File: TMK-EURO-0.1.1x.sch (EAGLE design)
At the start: 43 parts, among them IC1 TL082P, U2 IN, U5 IN, U6 IN, U7 THONKICONNOLD, X1 057-010-1

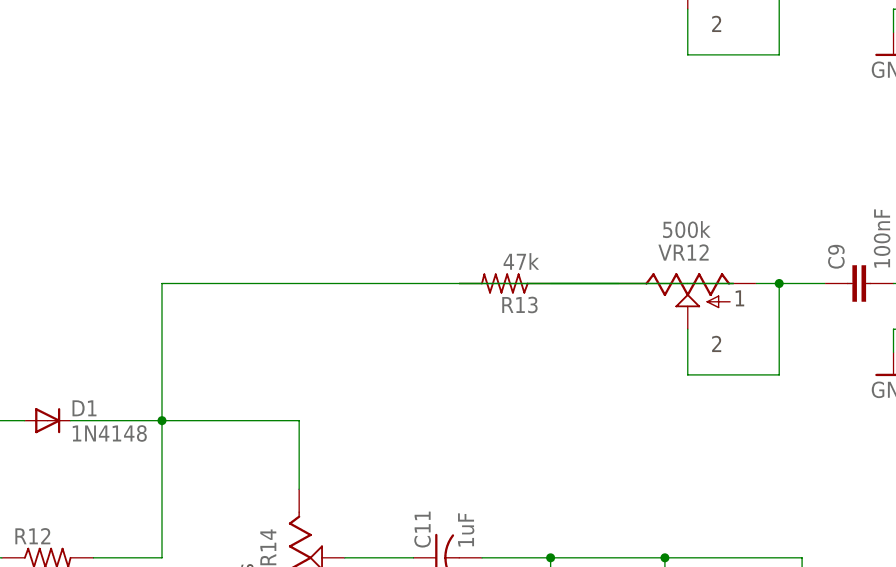
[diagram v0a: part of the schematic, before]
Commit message: Nets netjes
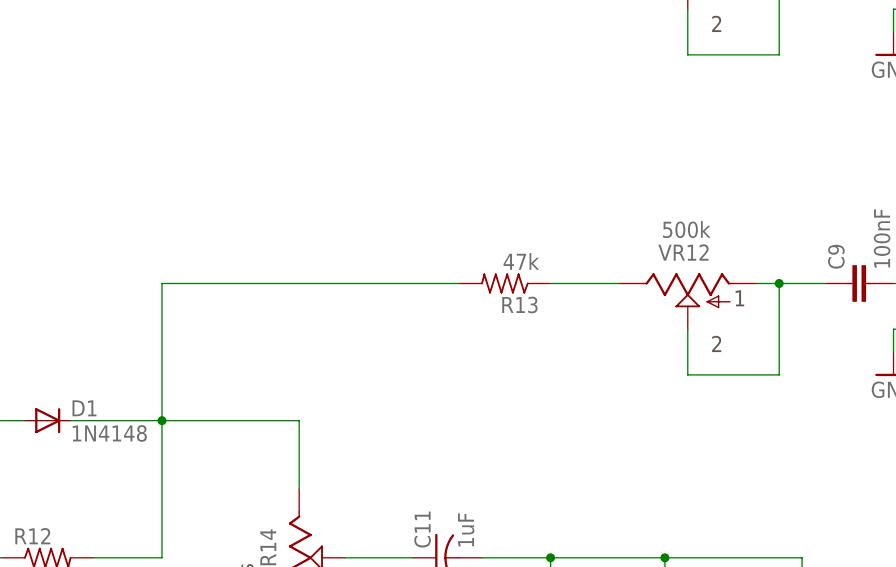
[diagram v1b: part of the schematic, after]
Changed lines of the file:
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@@
 <junction x="208.28" y="116.84"/>
 <wire x1="208.28" y1="116.84" x2="208.28" y2="132.08" width="0.1524" layer="91"/>
-<wire x1="208.28" y1="132.08" x2="246.38" y2="132.08" width="0.1524" layer="91"/>
-<wire x1="246.38" y1="132.08" x2="266.7" y2="132.08" width="0.1524" layer="91"/>
-<wire x1="266.7" y1="132.08" x2="271.78" y2="132.08" width="0.1524" layer="91"/>
 <pinref part="R13" gate="G$1" pin="2"/>
-<wire x1="271.78" y1="132.08" x2="241.3" y2="132.08" width="0.1524" layer="91"/>
+<wire x1="208.28" y1="132.08" x2="241.3" y2="132.08" width="0.1524" layer="91"/>
 </segment>
 </net>
@@
 </segment>
 </net>
-<net name="N$17" class="0">
-<segment>
-<pinref part="R13" gate="G$1" pin="1"/>
-<pinref part="VR12" gate="G$1" pin="E"/>
-<wire x1="251.46" y1="132.08" x2="259.08" y2="132.08" width="0.1524" layer="91"/>
-</segment>
-</net>
 <net name="N$26" class="2">
 <segment>
@@
 </segment>
 </net>
+<net name="N$4" class="0">
+<segment>
+<pinref part="R13" gate="G$1" pin="1"/>
+<pinref part="VR12" gate="G$1" pin="E"/>
+<wire x1="251.46" y1="132.08" x2="259.08" y2="132.08" width="0.1524" layer="91"/>
+</segment>
+</net>
 </nets>
 </sheet>
 </sheets>
-<errors>
-</errors>
 </schematic>
 </drawing>
